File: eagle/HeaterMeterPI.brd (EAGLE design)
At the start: 120 x 45.7 mm, 76 parts, among them IC1 OKI-78SR-5, IC2 ATmega328P, IC3 74HC595N, IC4 MCP1700-33, IC5 AD849X, J1 LCD, J2 PROBE, J4 PCC-SMP, J7 ICSP, J8 FTDI, J9 POW, Q1 BS170, Q2 BS170, Q3 FQU11P06TU, Q4 BS170, Q5 BS170, Y1 16MHz

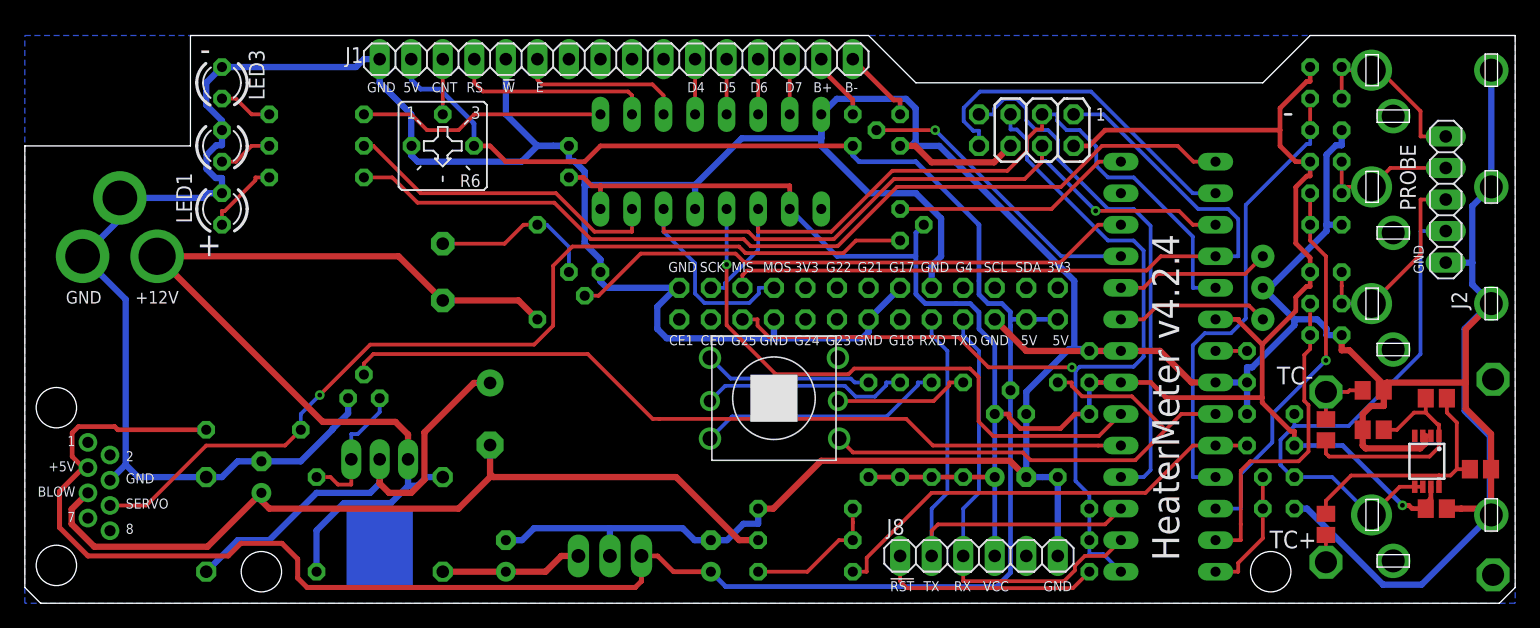
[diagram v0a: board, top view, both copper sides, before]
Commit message: [eagle] HeaterMeter v4.3 Main and LCD
v4.3.3 Release
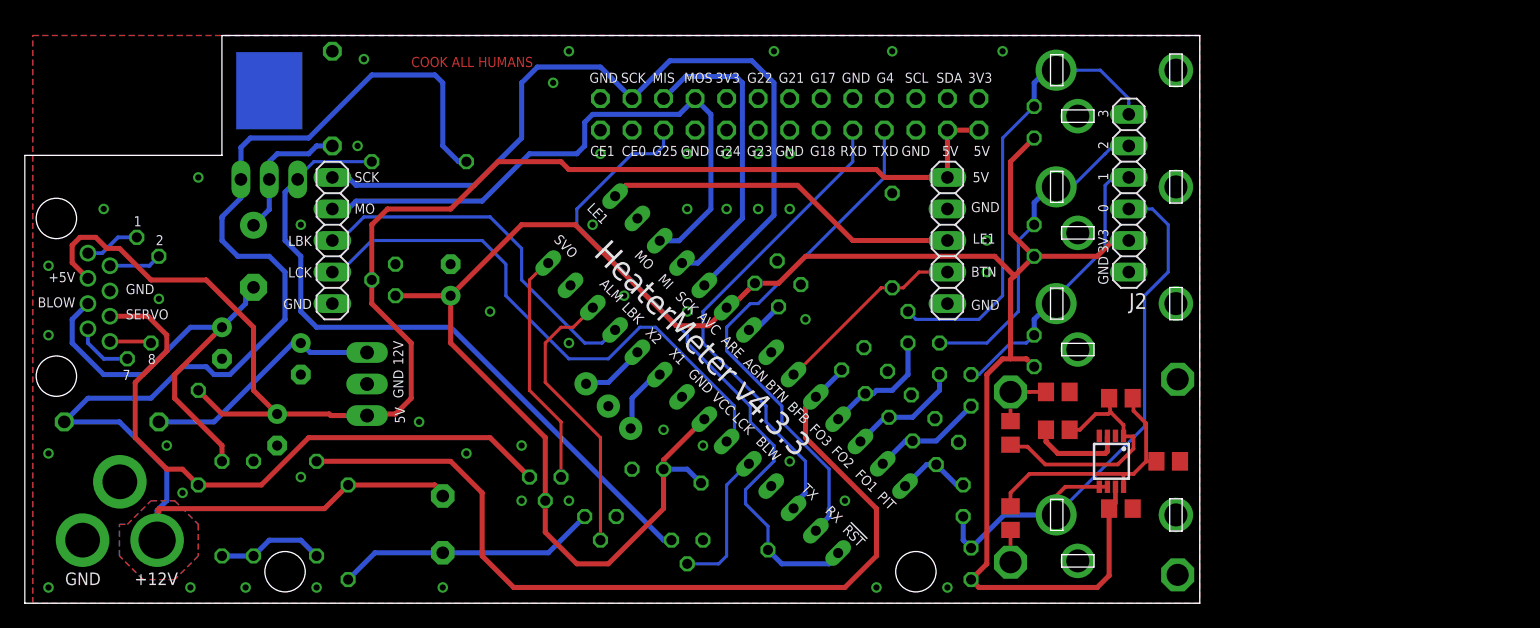
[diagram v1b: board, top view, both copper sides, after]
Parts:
- removed C10: 0.1u, resistor:C025-025X050
- removed IC3: 74HC595N, 74xx-us:DIL16
- removed J7: ICSP, pinhead:2X04
- removed J8: FTDI, pinhead:1X06
- removed LED1, LED2, LED3: GRN, led:LED3MM
- removed Q4: BS170, transistor-small-signal:SOT54E
- removed R10, R12, R15, R2: 390, resistor:0204/7
- removed R11: 4k7, resistor:0204/7
- removed R6: 10k, pot:CT6
- removed R7: 0, resistor:0204V
- removed R8: 680, resistor:0204/7
- removed R9: 2k2, resistor:0204/7
- removed S1: TACTILE-4, Bryan:TACT4
- added JP8: LCD2F, pinhead:1X05
- added U$1, U$2, U$3, U$4: THROUGH-HOLE, Bryan:PAD-032
- D3: value 1N4001 -> 1N5819
- J1: value LCD -> RPi; device pinhead:1X16 -> pinhead:2X13
- J2: device pinhead:1X05 -> pinhead:1X06
- JP1: value Pi -> LCD1F; device pinhead:2X13 -> pinhead:1X05
- moved Y1 53.6 mm to (46.4, 15.9), turned to 45 degrees
- moved IC4 50.7 mm to (29.2, 26.0), turned to 270 degrees
- moved C6 47.8 mm to (33.7, 26.0), turned to 90 degrees
- moved R13 47.1 mm to (15.2, 7.62), turned to 270 degrees
- moved R4 44.4 mm to (17.8, 7.62), turned to 90 degrees
- moved JP1 43.5 mm to (24.1, 29.2), flipped to the top, turned to 270 degrees
- moved C18 41.5 mm to (67.9, 17.8), turned to 135 degrees
- moved R19 39.7 mm to (22.9, 7.62), turned to 90 degrees
- moved C3 39.5 mm to (59.1, 26.7), turned to 135 degrees
- moved R22 38.4 mm to (70.5, 22.2), turned to 90 degrees
- moved C17 37.3 mm to (69.8, 15.9), turned to 135 degrees
- moved C1 36.5 mm to (49.5, 10.8), turned to 0 degrees
- moved C5 36.4 mm to (19.7, 14.0), turned to 270 degrees
- moved D2 35.8 mm to (24.1, 40.6)
- moved IC2 35.6 mm to (55.9, 18.4), turned to 45 degrees
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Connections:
- removed net BKLT: J1.15, R7.2
- removed net BKLT_GND: J1.16, Q4.D
- removed net D4: IC3.4, J1.11
- removed net D5: IC3.5, J1.12
- removed net D6: IC3.6, J1.13
- removed net D7: IC3.7, J1.14
- removed net E: IC3.3, J1.6
- removed net N$10: R11.1, S1.2
- removed net N$12: R9.1, S1.3
- removed net N$14: R2.2, S1.5
- removed net N$15: LED2.A, R10.2
- removed net N$17: C3.1, IC2.21
- removed net N$18: IC3.15, R10.1
- removed net N$19: IC3.1, R12.1
- removed net N$20: LED3.A, R12.2
- removed net N$24: LED1.A, R15.2
- removed net N$3: J1.3, R6.S
- removed net N$8: R8.1, S1.1
- removed net RS: IC3.2, J1.4
- new net OUT-1: JP2.1, U$3.P
- new net OUT-2: JP2.2, U$4.P
- new net OUT-7: JP2.7, U$2.P
- new net OUT-8: JP2.8, U$1.P
- net !IRQ: no longer J7.8
- net !RESET: now also J1.6; no longer C10.1, J7.6, JP1.6
- net !RF_SEL: no longer J7.7
- net +3V3: now also C3.1, J2.2; no longer C2.1, IC3.10, IC3.16, J7.1, J8.3, R11.2, R2.1, R8.2, R9.2
- net +5V: now also J1.24, J1.26, JP8.1; no longer J1.2, JP1.24, JP1.26, R6.E, R7.1
- net BUTTONS: now also JP8.4; no longer S1.4
- net FOOD1_P: now also J2.4; no longer J2.3
- net FOOD2_P: now also J2.5; no longer J2.4
- net FOOD3_P: now also J2.6; no longer J2.5
- net GND: now also J1.14, J1.17, J1.22, J1.8, JP1.5, JP8.2, JP8.5; no longer IC3.13, IC3.8, J1.5, J7.5, J8.1, JP1.1, JP1.14, JP1.15, JP1.17, JP1.22, JP1.8, LED1.K, LED2.K, LED3.K, Q4.S, R6.A
- net LCD_BKLT: now also JP1.3; no longer Q4.G
- net LCD_CLK: now also JP1.4; no longer IC3.12
- net LED1: now also JP8.3; no longer R15.1
- net MISO: now also J1.5; no longer J7.2, JP1.5
- net MOSI: now also J1.7, JP1.2; no longer IC3.14, J7.3, JP1.7
- net N$2: now also C2.1, IC2.21; no longer C10.2, J8.6
- net PIT_P: now also J2.3; no longer J2.2
- net RX: now also J1.20; no longer J8.4, JP1.20
- net SCK: now also J1.3, JP1.1; no longer IC3.11, J7.4, JP1.3
- net TX: now also J1.18; no longer J8.5, JP1.18
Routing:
- net GND: track 490.3 -> 7.60 mm, vias 0 -> 50
- net +5V: track 192.8 -> 119.0 mm
- net BLOWER: track 65.2 -> 11.7 mm
- net LED1: track 74.7 -> 29.1 mm
- net N$1: track 11.2 -> 55.7 mm
- net !IRQ: track 42.6 -> 0.00 mm
- net MISO: track 61.3 -> 24.6 mm
- net +12V_FB: track 36.6 -> 72.7 mm
- net +12V_BLW: track 67.6 -> 37.0 mm
- net +12V: track 78.3 -> 108.9 mm
- net !RF_SEL: track 28.1 -> 0.00 mm
- net FOOD3: track 37.6 -> 9.65 mm
- net BUTTONS: track 43.0 -> 15.8 mm
- net N$18: track 26.3 -> 0.00 mm
- net !RESET: track 78.6 -> 52.6 mm, vias 1 -> 0
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- added copper zone on layer 1, net +12V
- added copper zone on layer 16, net +12V
- added copper zone on layer 1, net GND
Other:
- board size 120 x 45.7 mm -> 94.6 x 45.7 mm
- board text added: "0"
- board text added: "12V"
- board text added: "3"
- board text added: "AGN"
- board text added: "ALM"
- board text added: "ARE"
- board text added: "AVC"
- board text added: "BFB"
- board text added: "BLW"
- board text added: "BTN"
- board text added: "COOK ALL HUMANS"
- board text added: "FO1"
- board text added: "FO2"
- board text added: "FO3"
- board text added: "HeaterMeter v4.3.3"
- board text added: "LBK"
- board text added: "LCK"
- board text added: "LE1"
- board text added: "MI"
- board text added: "MO"
- board text added: "PIT"
- board text added: "SVO"
- board text added: "X1"
- board text added: "X2"
- board text removed: "!W"
- board text removed: "+"
- board text removed: "-"
- board text removed: "0.1u"
- board text removed: "0.750" From Edge"
- board text removed: "0.775" From Edge"
- board text removed: "4.725" x 1.780""
- board text removed: "B+"
- board text removed: "B-"
- board text removed: "CNT"
- board text removed: "D4"
- board text removed: "D5"
- board text removed: "D6"
- board text removed: "D7"
- board text removed: "E"
- board text removed: "HeaterMeter v4.2.4"
- board text removed: "Overall Dimensions"
- board text removed: "RS"
- board text removed: "TC+"
- board text removed: "TC-"
